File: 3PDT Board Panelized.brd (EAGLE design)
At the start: 77.1 x 92.7 mm, 0 parts

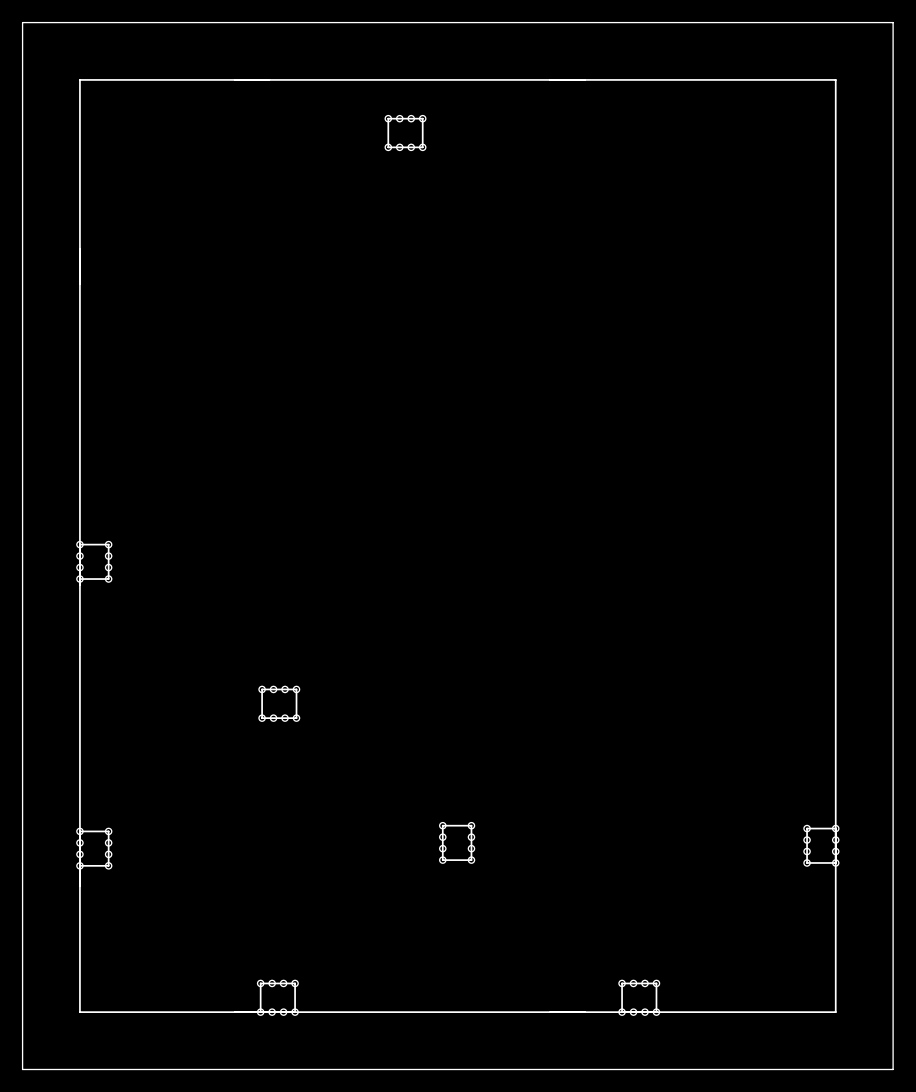
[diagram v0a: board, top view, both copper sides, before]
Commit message: Commit Seeed board and backup files
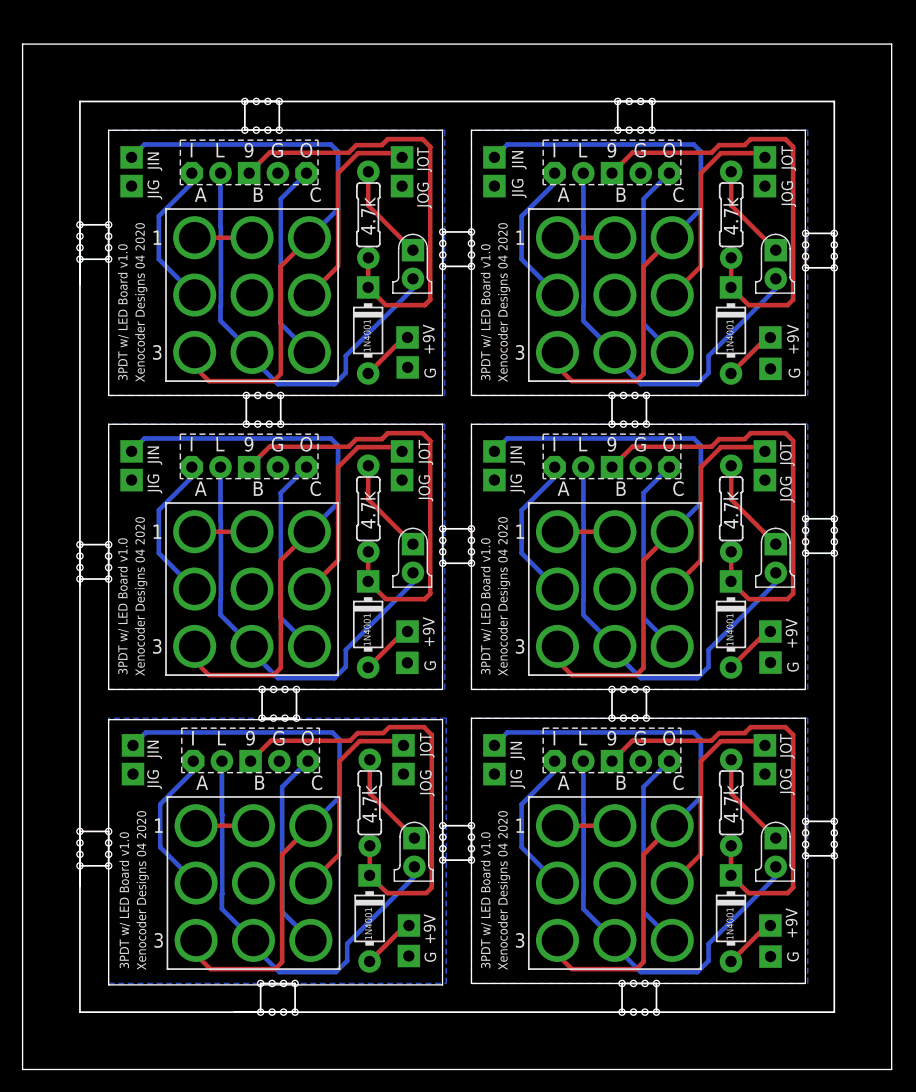
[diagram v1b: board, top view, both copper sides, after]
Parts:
- added +9V, +9V1, +9V2, +9V3, +9V4, +9V5: +9V(T), mb_supply:SQUARE
- added D1, D11, D3, D5, D7, D9: 1N4001, mb_diodes:DO41-3
- added D10, D12, D2, D4, D6, D8: LED3MM, mb_diodes:LED3MM
- added G, G2, G3, G4, G5, JIG, JIG1, JIG2, JIG3, JIG4, JIG5, JOG, JOG1, JOG2, JOG3, JOG4, JOG5: GND(T), mb_supply:SQUARE
- added G1: G, mb_supply:SQUARE
- added JIN, JIN1, JIN2, JIN3, JIN4, JIN5, JOT, JOT1, JOT2, JOT3, JOT4, JOT5: (no value), mb_supply:SQUARE
- added R1, R2, R3, R4, R5, R6: 4.7k, mb_resistors:R0207/3
- added SW1, SW2, SW3, SW4, SW5, SW6: 3PDT, mb_switches:3PDT
- added U$1, U$2, U$3, U$4, U$5, U$6: BOARDLINK, xc_library:BOARDLINK
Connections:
- new net +9V: +9V.1, D1.A
- new net +9V1: +9V1.1, D3.A
- new net +9V2: +9V2.1, D5.A
- new net +9V3: +9V3.1, D7.A
- new net +9V4: +9V4.1, D9.A
- new net +9V5: +9V5.1, D11.A
- new net A: D1.C, R1.2, U$1.3
- new net A1: D3.C, R2.2, U$2.3
- new net A2: D5.C, R3.2, U$3.3
- new net A3: D7.C, R4.2, U$4.3
- new net A4: D9.C, R5.2, U$5.3
- new net A5: D11.C, R6.2, U$6.3
- new net B: D2.K, SW2.B3, U$1.2
- new net B1: D4.K, SW1.B3, U$2.2
- new net B2: D6.K, SW3.B3, U$3.2
- new net B3: D8.K, SW4.B3, U$4.2
- new net B4: D10.K, SW5.B3, U$5.2
- new net B5: D12.K, SW6.B3, U$6.2
- new net GND: G.1, JIG.1, JOG.1, SW2.B2, U$1.4
- new net GND1: G1.1, JIG1.1, JOG1.1, SW1.B2, U$2.4
- new net GND2: G2.1, JIG2.1, JOG2.1, SW3.B2, U$3.4
- new net GND3: G3.1, JIG3.1, JOG3.1, SW4.B2, U$4.4
- new net GND4: G4.1, JIG4.1, JOG4.1, SW5.B2, U$5.4
- new net GND5: G5.1, JIG5.1, JOG5.1, SW6.B2, U$6.4
- new net N$1: JOT1.1, SW1.C2
- new net N$10: SW1.A2, U$2.1
- new net N$11: SW1.C3, U$2.5
- new net N$12: D4.A, R2.1
- new net N$13: JOT2.1, SW3.C2
- new net N$14: JIN2.1, SW3.A3, SW3.C1
- new net N$15: SW3.A1, SW3.B1
- new net N$16: SW3.A2, U$3.1
- new net N$17: SW3.C3, U$3.5
- new net N$18: D6.A, R3.1
- new net N$19: JOT3.1, SW4.C2
- new net N$2: JOT.1, SW2.C2
- new net N$20: JIN3.1, SW4.A3, SW4.C1
- new net N$21: SW4.A1, SW4.B1
- new net N$22: SW4.A2, U$4.1
- new net N$23: SW4.C3, U$4.5
- new net N$24: D8.A, R4.1
- new net N$25: JOT4.1, SW5.C2
- new net N$26: JIN4.1, SW5.A3, SW5.C1
- new net N$27: SW5.A1, SW5.B1
- new net N$28: SW5.A2, U$5.1
- new net N$29: SW5.C3, U$5.5
- new net N$3: SW2.A1, SW2.B1
- new net N$30: D10.A, R5.1
- new net N$31: JOT5.1, SW6.C2
- new net N$32: JIN5.1, SW6.A3, SW6.C1
- new net N$33: SW6.A1, SW6.B1
- new net N$34: SW6.A2, U$6.1
- new net N$35: SW6.C3, U$6.5
- new net N$36: D12.A, R6.1
- new net N$4: JIN.1, SW2.A3, SW2.C1
- new net N$5: SW2.A2, U$1.1
- new net N$6: SW2.C3, U$1.5
- new net N$7: D2.A, R1.1
- new net N$8: JIN1.1, SW1.A3, SW1.C1
- new net N$9: SW1.A1, SW1.B1
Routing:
- net N$26: track 0.00 -> 50.5 mm
- net N$20: track 0.00 -> 50.5 mm
- net N$14: track 0.00 -> 50.5 mm
- net N$32: track 0.00 -> 50.5 mm
- net N$4: track 0.00 -> 50.5 mm
- net N$8: track 0.00 -> 50.5 mm
- net A1: track 0.00 -> 40.1 mm
- net A5: track 0.00 -> 40.1 mm
- net A4: track 0.00 -> 40.1 mm
- net A3: track 0.00 -> 40.1 mm
- net A: track 0.00 -> 40.1 mm
- net A2: track 0.00 -> 40.1 mm
- net B4: track 0.00 -> 38.0 mm
- net B3: track 0.00 -> 38.0 mm
- net B2: track 0.00 -> 38.0 mm
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- added copper zone on layer 16, net GND
- added copper zone on layer 16, net GND1
- added copper zone on layer 16, net GND2
- added copper zone on layer 16, net GND3
- added copper zone on layer 16, net GND4
- added copper zone on layer 16, net GND5
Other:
- board size 77.1 x 92.7 mm -> 77 x 90.8 mm
- board text added: "+9V"
- board text added: "3PDT w/ LED Board v1.0"
- board text added: "G"
- board text added: "JIG"
- board text added: "JIN"
- board text added: "JOG"
- board text added: "JOT"
- board text added: "Xenocoder Designs 04 2020"
